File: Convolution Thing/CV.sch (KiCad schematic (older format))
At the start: 82 parts, among them J10 In CV 4, J11 In CV 5, J12 In CV 6, J13 In CV 7, J14 In CV 8, J7 In CV 1, J8 In CV 2, J9 In CV 3, U5 LTC2309_TSSOP, U6 MCP6004, U7 MCP6004, U8 LM4040DBZ-2.5, U9 LM4040DBZ-2.5

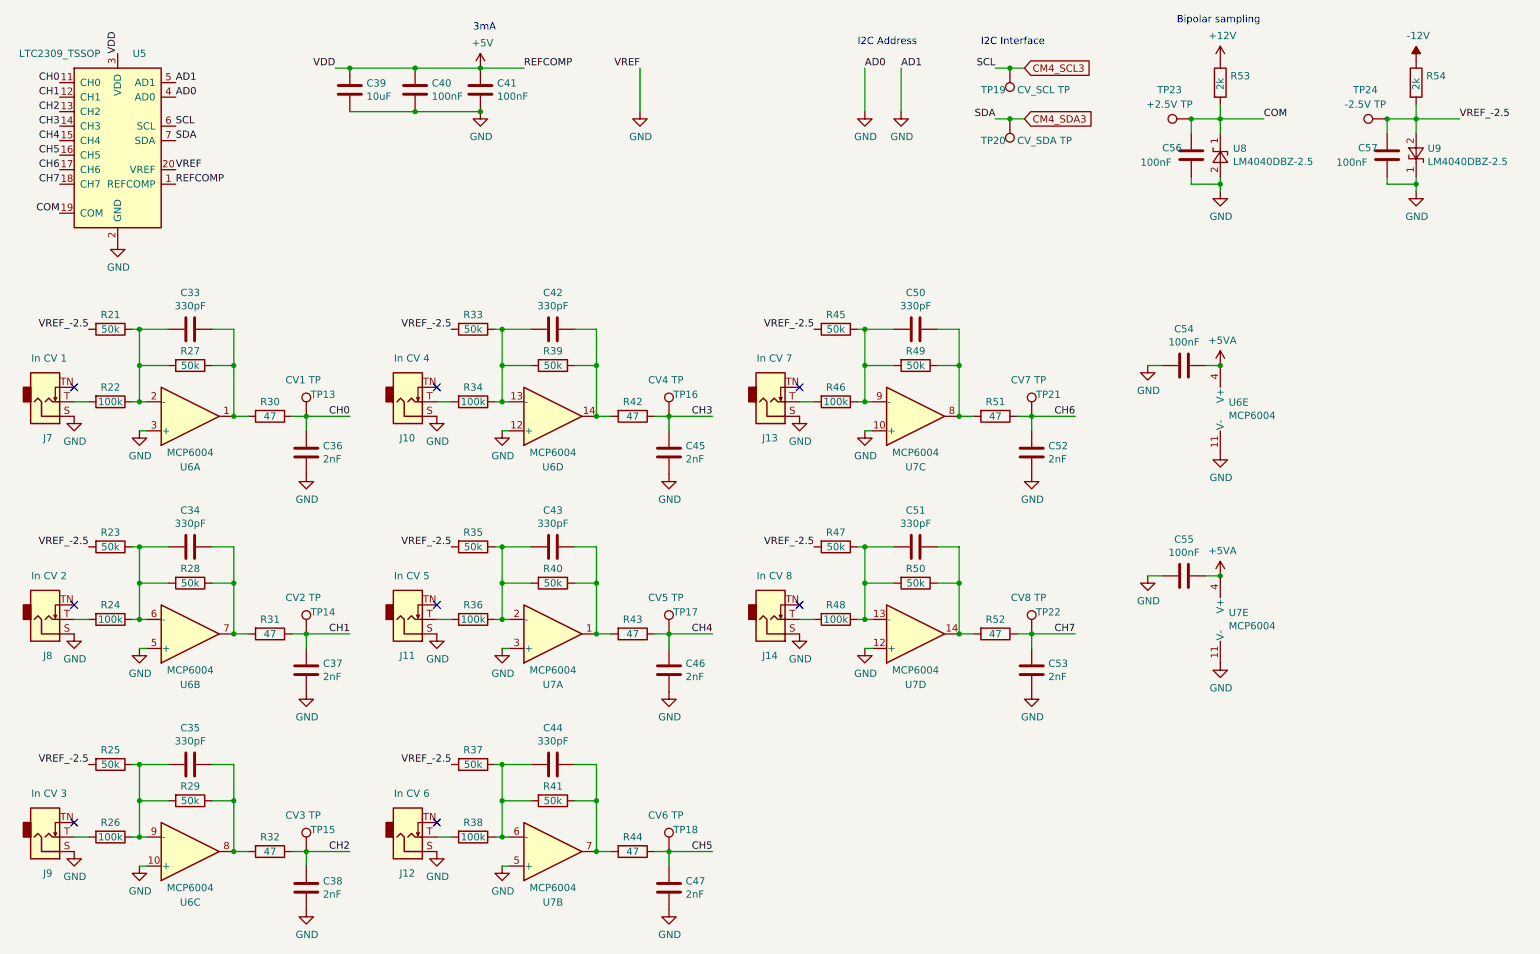
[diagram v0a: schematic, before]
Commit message: PCB layout
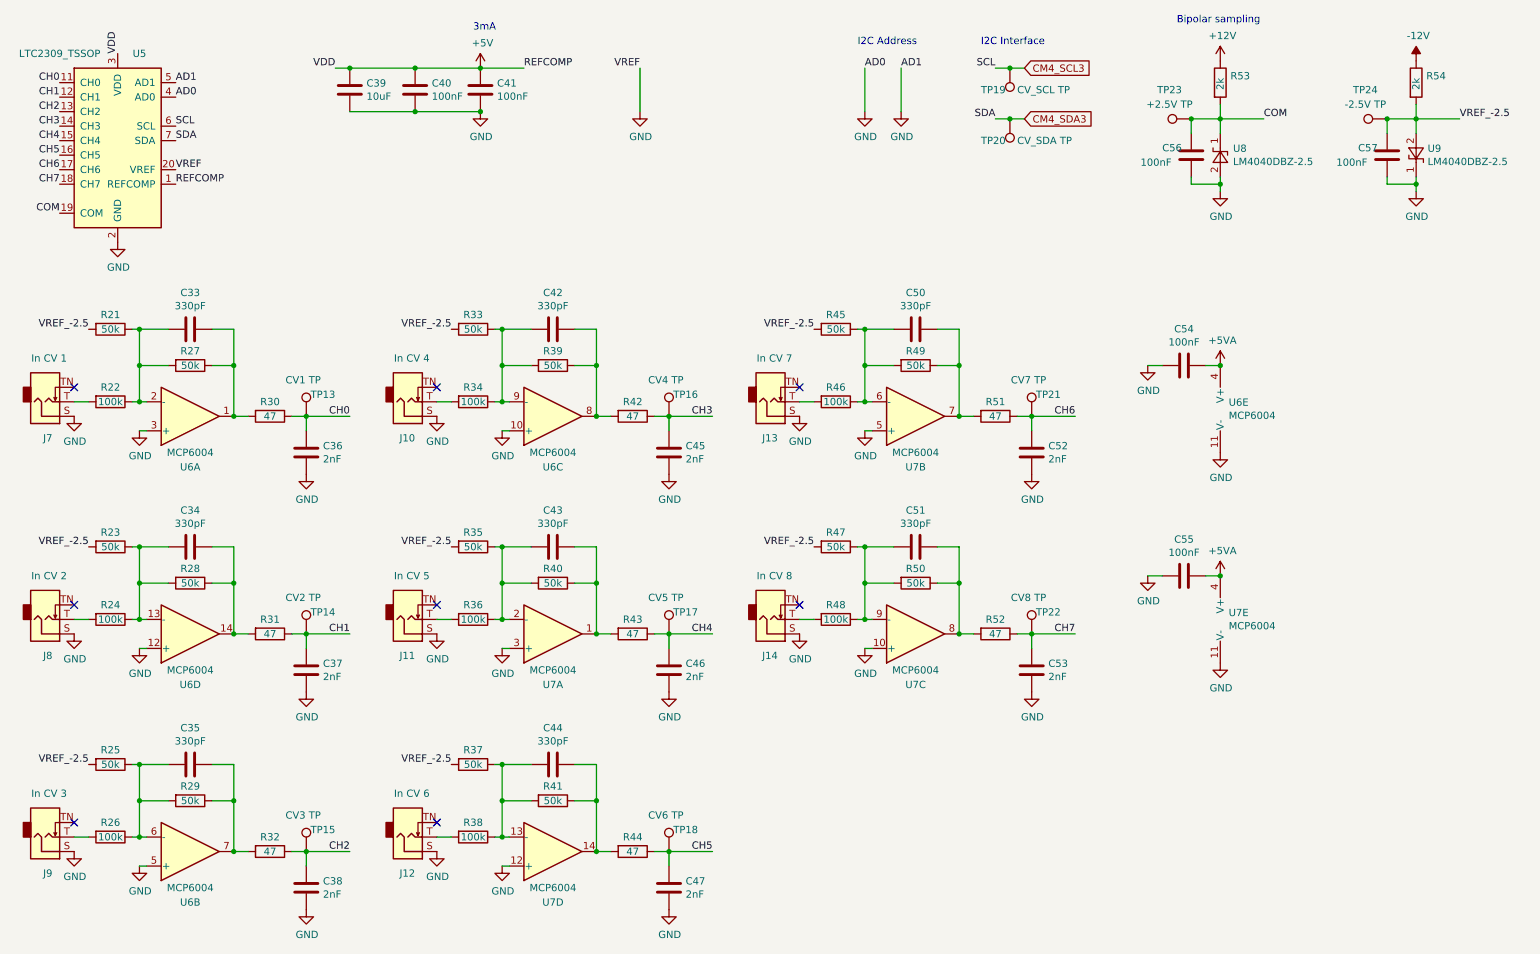
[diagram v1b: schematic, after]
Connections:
- net GND: now also U6.10 (+), U6.12 (+), U6.5 (+), U7.10 (+), U7.12 (+), U7.5 (+); no longer U6.10 (+), U6.12 (+), U6.5 (+), U7.10 (+), U7.12 (+), U7.5 (+)
- net at C34.2, R23.1, R24.1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: now also U6.13 (-); no longer U6.6 (-)
- net at C34.1, R28.1, R31.2: now also U6.14; no longer U6.7
- net at C35.1, R29.1, R32.2: now also U6.7; no longer U6.8
- net at C35.2, R25.1, R26.1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: now also U6.6 (-); no longer U6.9 (-)
- net at C42.2, R33.1, R34.1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: now also U6.9 (-); no longer U6.13 (-)
- net at C42.1, R39.1, R42.2: now also U6.8; no longer U6.14
- net at C44.2, R37.1, R38.1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: now also U7.13 (-); no longer U7.6 (-)
- net at C44.1, R41.1, R44.2: now also U7.14; no longer U7.7
- net at C50.1, R49.1, R51.2: now also U7.7; no longer U7.8
- net at C50.2, R45.1, R46.1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: now also U7.6 (-); no longer U7.9 (-)
- net at C51.2, R47.1, R48.1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: now also U7.9 (-); no longer U7.13 (-)
- net at C51.1, R50.1, R52.2: now also U7.8; no longer U7.14
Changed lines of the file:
@@
 $Comp
 L Amplifier_Operational:MCP6004 U6
-U 2 1 6112EF95
+U 4 1 6112EF95
 P 1900 4900
 F 0 "U6" H 1900 5250 50  0000 C CNN
@@
 F 2 "Package_SO:SOIC-14_3.9x8.7mm_P1.27mm" H 1850 5000 50  0001 C CNN
 F 3 "http://ww1.microchip.com/downloads/en/DeviceDoc/21733j.pdf" H 1950 5100 50  0001 C CNN
-	2    1900 4900
+	4    1900 4900
 	1    0    0    1
 $EndComp
@@
 $Comp
 L Amplifier_Operational:MCP6004 U6
-U 3 1 61134A88
+U 2 1 61134A88
 P 1900 6400
 F 0 "U6" H 1900 6750 50  0000 C CNN
@@
 F 2 "Package_SO:SOIC-14_3.9x8.7mm_P1.27mm" H 1850 6500 50  0001 C CNN
 F 3 "http://ww1.microchip.com/downloads/en/DeviceDoc/21733j.pdf" H 1950 6600 50  0001 C CNN
-	3    1900 6400
+	2    1900 6400
 	1    0    0    1
 $EndComp
@@
 $Comp
 L Amplifier_Operational:MCP6004 U6
-U 4 1 611437DD
+U 3 1 611437DD
 P 4400 3400
 F 0 "U6" H 4400 3750 50  0000 C CNN
@@
 F 2 "Package_SO:SOIC-14_3.9x8.7mm_P1.27mm" H 4350 3500 50  0001 C CNN
 F 3 "http://ww1.microchip.com/downloads/en/DeviceDoc/21733j.pdf" H 4450 3600 50  0001 C CNN
-	4    4400 3400
+	3    4400 3400
 	1    0    0    1
 $EndComp
@@
 CH4
 $Comp
-L Amplifier_Operational:MCP6004 U7
-U 1 1 6114382C
-P 4400 4900
-F 0 "U7" H 4400 5250 50  0000 C CNN
-F 1 "MCP6004" H 4400 5150 50  0000 C CNN
-F 2 "Package_SO:SOIC-14_3.9x8.7mm_P1.27mm" H 4350 5000 50  0001 C CNN
-F 3 "http://ww1.microchip.com/downloads/en/DeviceDoc/21733j.pdf" H 4450 5100 50  0001 C CNN
-	1    4400 4900
-	1    0    0    1
-$EndComp
-$Comp
 L Device:R R36
 U 1 1 61143832
@@
 $Comp
 L Amplifier_Operational:MCP6004 U7
-U 2 1 6114387B
+U 4 1 6114387B
 P 4400 6400
 F 0 "U7" H 4400 6750 50  0000 C CNN
@@
 F 2 "Package_SO:SOIC-14_3.9x8.7mm_P1.27mm" H 4350 6500 50  0001 C CNN
 F 3 "http://ww1.microchip.com/downloads/en/DeviceDoc/21733j.pdf" H 4450 6600 50  0001 C CNN
-	2    4400 6400
+	4    4400 6400
 	1    0    0    1
 $EndComp
@@
 $Comp
 L Amplifier_Operational:MCP6004 U7
-U 3 1 61156AFF
+U 2 1 61156AFF
 P 6900 3400
 F 0 "U7" H 6900 3750 50  0000 C CNN
@@
 F 2 "Package_SO:SOIC-14_3.9x8.7mm_P1.27mm" H 6850 3500 50  0001 C CNN
 F 3 "http://ww1.microchip.com/downloads/en/DeviceDoc/21733j.pdf" H 6950 3600 50  0001 C CNN
-	3    6900 3400
+	2    6900 3400
 	1    0    0    1
 $EndComp
@@
 $Comp
 L Amplifier_Operational:MCP6004 U7
-U 4 1 61156B4E
+U 3 1 61156B4E
 P 6900 4900
 F 0 "U7" H 6900 5250 50  0000 C CNN
@@
 F 2 "Package_SO:SOIC-14_3.9x8.7mm_P1.27mm" H 6850 5000 50  0001 C CNN
 F 3 "http://ww1.microchip.com/downloads/en/DeviceDoc/21733j.pdf" H 6950 5100 50  0001 C CNN
-	4    6900 4900
+	3    6900 4900
 	1    0    0    1
 $EndComp
@@
 Wire Wire Line
 	4200 1000 3900 1000
+$Comp
+L Amplifier_Operational:MCP6004 U7
+U 1 1 6114382C
+P 4400 4900
+F 0 "U7" H 4400 5250 50  0000 C CNN
+F 1 "MCP6004" H 4400 5150 50  0000 C CNN
+F 2 "Package_SO:SOIC-14_3.9x8.7mm_P1.27mm" H 4350 5000 50  0001 C CNN
+F 3 "http://ww1.microchip.com/downloads/en/DeviceDoc/21733j.pdf" H 4450 5100 50  0001 C CNN
+	1    4400 4900
+	1    0    0    1
+$EndComp
 $EndSCHEMATC
